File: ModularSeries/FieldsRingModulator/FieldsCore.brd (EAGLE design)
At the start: 44 x 65 mm, 39 parts

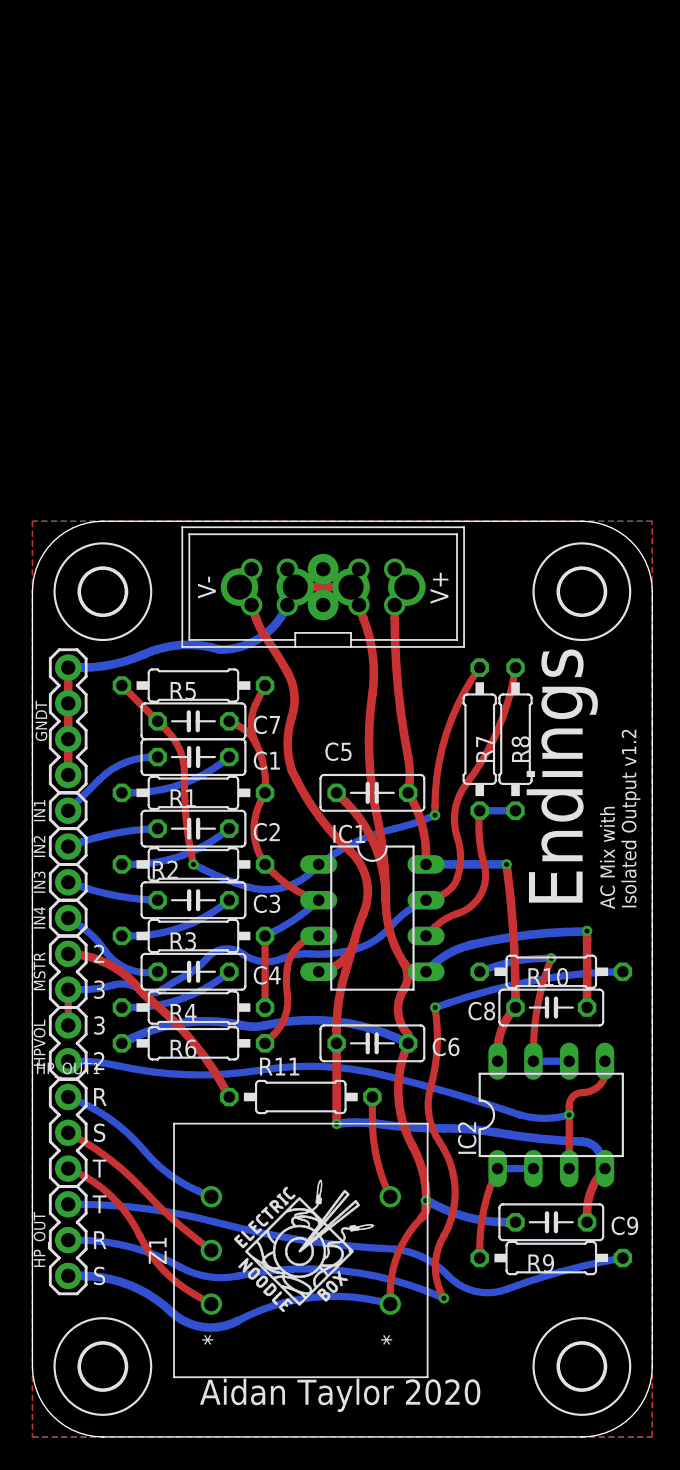
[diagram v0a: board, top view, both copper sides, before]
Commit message: Fields added and various updates to designs
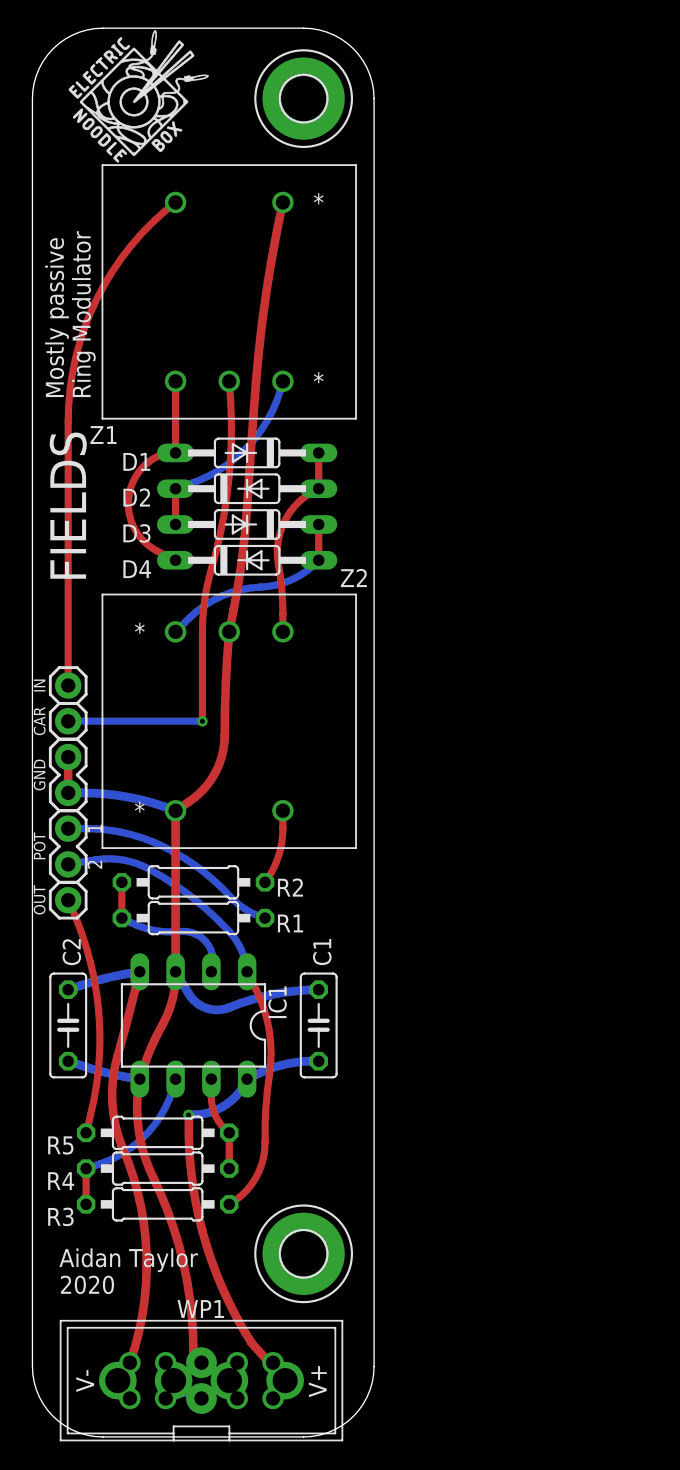
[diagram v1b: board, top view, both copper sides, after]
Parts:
- removed C3, C4: 220nF, rcl:C050-025X075
- removed C5, C6, C8, C9: 100nF, rcl:C050-025X075
- removed C7: 22pF, rcl:C050-025X075
- removed GNDT: 4XWIREPAD, ElectricNoodleBox:1X04
- removed H3, H4: MOUNT-HOLE3.2, holes:3,2
- removed HPVOL, MSTR: A100K, ElectricNoodleBox:1X02
- removed HP_OUT, HP_OUT1: 3XWIREPAD, ElectricNoodleBox:1X03
- removed IC2: (no value), ElectricNoodleBox:DIL08
- removed IN1, IN2, IN3, IN4: B100K, ElectricNoodleBox:1X01
- removed R10, R9: 75Ω, rcl:0207/10
- removed R11: 1K, rcl:0207/10
- removed R6, R7: 100K, rcl:0207/10
- removed R8: 12K, rcl:0207/10
- added CAR, IN, OUT: 1XWIREPAD, ElectricNoodleBox:1X01
- added D1, D2, D3, D4: (no value), diode:DO35-10
- added GND, POT: 2XWIREPAD, ElectricNoodleBox:1X02
- added Z2: (no value), ElectricNoodleBox:Z1604_TRANSFORMER
- C1, C2: value 220nF -> 100nF
- H1, H2: value MOUNT-HOLE3.2 -> MOUNT-PAD-ROUND3.2; device holes:3,2 -> holes:3,2-PAD
- R1, R2, R3, R4: value 100K -> 10K
- R5: value 47K -> 100Ω
- moved H2 92.1 mm to (19.2, 95.0)
- moved U$2 82.8 mm to (11.4, 90.2)
- moved U$1 82.4 mm to (2.54, 90.2)
- moved Z1 68.2 mm to (14.0, 81.3), turned to 0 degrees
- moved WP1 57.0 mm to (12.0, 4.00)
- moved R5 31.9 mm to (8.89, 21.6), turned to 180 degrees
- moved C1 21.0 mm to (20.3, 29.2), turned to 90 degrees
- moved R3 19.2 mm to (8.89, 16.5), turned to 180 degrees
- moved C2 16.6 mm to (2.54, 29.2), turned to 90 degrees
- moved H1 16.3 mm to (19.2, 13.0)
- moved IC1 14.8 mm to (11.4, 29.2), turned to 180 degrees
- moved R4 11.7 mm to (8.89, 19.1)
- moved R1 6.35 mm to (11.4, 39.4), turned to 180 degrees
- moved R2 3.81 mm to (11.4, 36.8)
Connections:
- removed net HP_VOLOUT: HPVOL.2, IC2.3, IC2.5
- removed net N$15: HP_OUT1.1, Z1.T6
- removed net N$16: HP_OUT1.2, Z1.T5
- removed net N$17: HP_OUT1.3, Z1.T4
- removed net N$18: IC2.1, IC2.2, R9.1
- removed net N$19: HP_OUT.1, R9.2
- removed net N$20: IC2.6, IC2.7, R10.1
- removed net N$21: HP_OUT.2, R10.2
- removed net N$22: R11.2, Z1.T1
- removed net N$9: C2.2, R2.1
- net +12V: now also C1.1; no longer C5.1, C8.1, IC2.8
- net -12V: now also C2.2; no longer C6.2, C9.2, IC2.4
- net AGND: now also C1.2, C2.1, GND.1, GND.2, IC1.3, Z2.T3, Z2.T5; no longer C5.2, C6.1, C8.2, C9.1, GNDT.1, GNDT.2, GNDT.3, GNDT.4, HP_OUT.3, R6.2
- net N$1: now also D1.A, D4.C, Z1.T6; no longer C4.1, IN4.1
- net N$10: now also POT.1, R2.2; no longer C3.2, R3.1
- net N$11: now also IC1.1, POT.2, R3.1; no longer C4.2, R4.1
- net N$12: now also IC1.6, R3.2, R4.1; no longer C2.1, IN2.1
- net N$13: now also IC1.7, R4.2, R5.1; no longer C1.1, IN1.1
- net N$14: now also OUT.1, R5.2; no longer MSTR.2, R11.1
- net N$2: now also D1.C, D2.A, Z2.T6; no longer C7.1, IC1.2, R1.2, R2.2, R3.2, R4.2, R5.2
- net N$3: now also D2.C, D3.A, Z1.T4; no longer C7.2, IC1.1, R5.1, R7.1
- net N$4: now also D3.C, D4.A, Z2.T4; no longer IC1.6, R7.2, R8.1
- net N$5: now also CAR.1, Z1.T5; no longer HPVOL.1, IC1.7, MSTR.1, R8.2
- net N$6: now also R1.1, Z2.T1; no longer C3.1, IN3.1
- net N$7: now also IC1.2, R1.2, R2.1; no longer IC1.3, R6.1
- net N$8: now also IN.1, Z1.T1; no longer C1.2, R1.1
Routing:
- net N$21: track 61.5 -> 0.00 mm, vias 2 -> 0
- net HP_VOLOUT: track 44.5 -> 0.00 mm, vias 1 -> 0
- net N$19: track 40.4 -> 0.00 mm
- net AGND: track 165.7 -> 127.0 mm, vias 2 -> 0
- net -12V: track 69.8 -> 36.3 mm, vias 1 -> 0
- net N$3: track 43.7 -> 13.4 mm, vias 2 -> 0
- net N$8: track 8.07 -> 36.1 mm
- net N$11: track 8.07 -> 33.6 mm
- net N$2: track 29.8 -> 13.4 mm
- net N$20: track 15.1 -> 0.00 mm, vias 1 -> 0
- net N$5: track 48.4 -> 33.8 mm, vias 0 -> 1
- net N$17: track 14.0 -> 0.00 mm
- net N$16: track 13.2 -> 0.00 mm
- net N$15: track 12.4 -> 0.00 mm
- net N$18: track 9.03 -> 0.00 mm
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- removed copper zone on layer 1, net AGND
- removed copper zone on layer 16, net AGND
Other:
- board size 44 x 65 mm -> 24.2 x 100 mm
- board text added: "1"
- board text added: "FIELDS"
- board text added: "Mostly passive Ring Modulator"
- board text removed: "3"
- board text removed: "AC Mix with Isolated Output v1.2"
- board text removed: "Endings"
- board text removed: "R"
- board text removed: "S"
- board text removed: "T"
